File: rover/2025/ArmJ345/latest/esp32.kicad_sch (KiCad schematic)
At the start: 15 parts, among them SW1 SW-PTS815SJM250SMTRLFS, SW2 SW-PTS815SJM250SMTRLFS, U7 ESP32-S3-WROVER

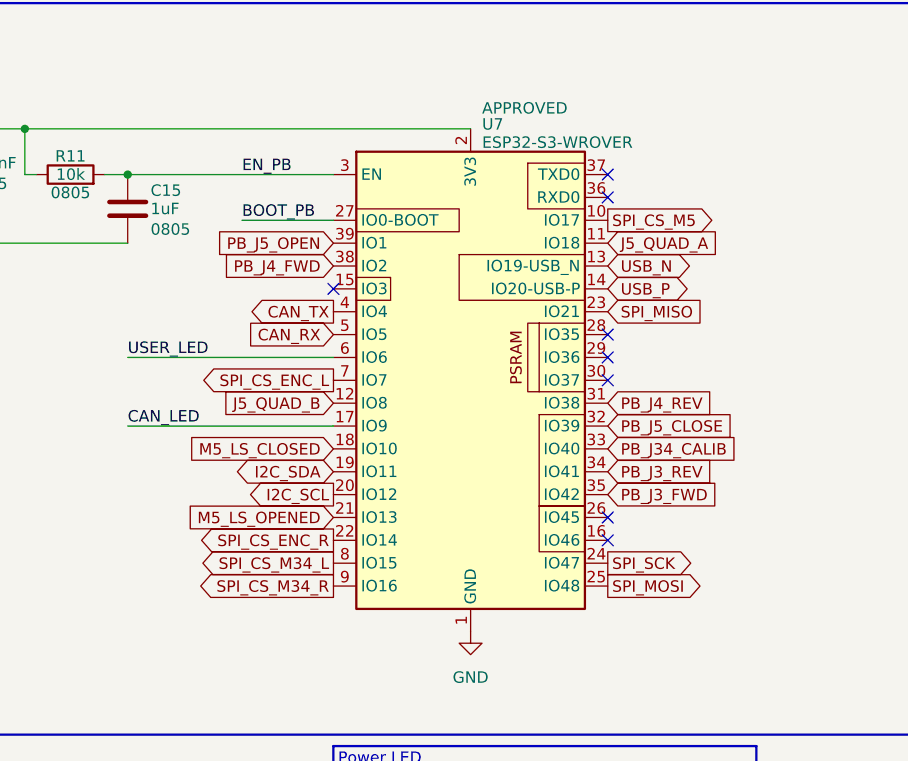
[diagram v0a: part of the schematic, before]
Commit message: armj345 fixes
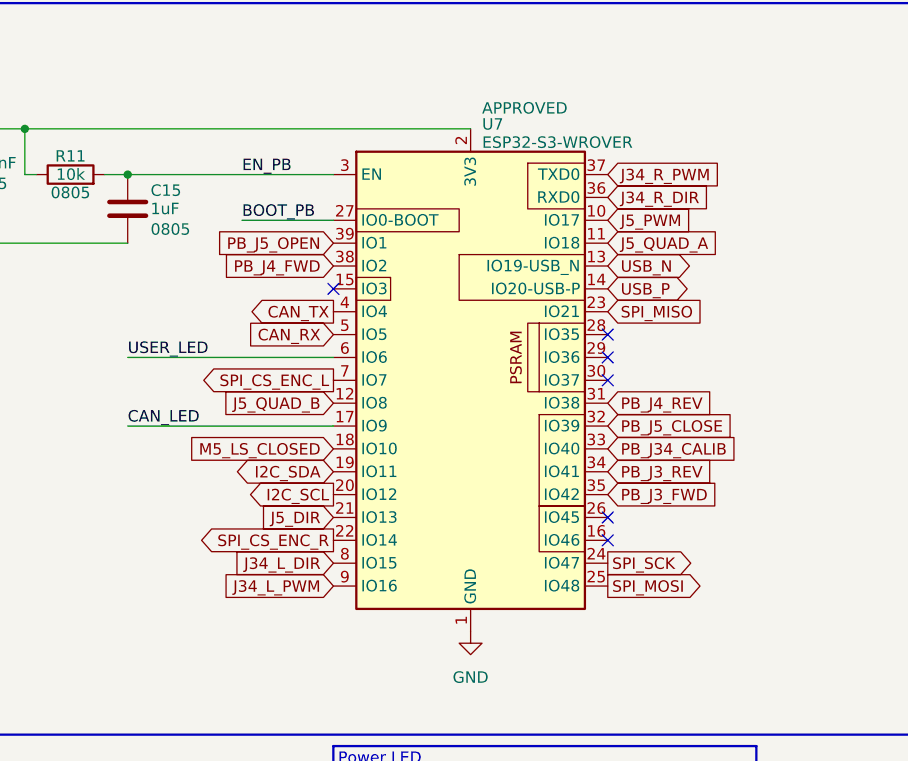
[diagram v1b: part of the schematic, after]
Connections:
- net J34_R_DIR: now reaches U7.36 (RXD0)
- net J34_R_PWM: now reaches U7.37 (TXD0)
- net M5_LS_OPENED renamed J5_DIR
- net SPI_CS_M34_L renamed J34_L_DIR
- net SPI_CS_M34_R renamed J34_L_PWM
- net SPI_CS_M5 renamed J5_PWM
- no-connect marks 8 -> 6
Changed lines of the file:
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@@
-	)
-	(no_connect
-		(at 116.84 31.75)
-	)
-	(no_connect
-		(at 116.84 34.29)
 	)
 	(no_connect
@@
 		)
 	)
-	(global_label "SPI_CS_M5"
-		(shape output)
+	(global_label "J5_PWM"
+		(shape input)
 		(at 116.84 36.83 0)
 		(fields_autoplaced yes)
@@
 		)
 		(property "Intersheetrefs" "${INTERSHEET_REFS}"
-			(at 129.9851 36.83 0)
+			(at 127.1427 36.83 0)
 			(effects
 				(font
@@
 		)
 	)
+	(global_label "J34_L_PWM"
+		(shape input)
+		(at 86.36 77.47 180)
+		(fields_autoplaced yes)
+		(effects
+			(font
+				(size 1.27 1.27)
+			)
+			(justify right)
+		)
+		(property "Intersheetrefs" "${INTERSHEET_REFS}"
+			(at 72.8521 77.47 0)
+			(effects
+				(font
+					(size 1.27 1.27)
+				)
+				(justify right)
+				(hide yes)
+			)
+		)
+	)
 	(global_label "SPI_CS_ENC_L"
 		(shape output)
@@
 		)
 	)
+	(global_label "J5_DIR"
+		(shape input)
+		(at 86.36 69.85 180)
+		(fields_autoplaced yes)
+		(effects
+			(font
+				(size 1.27 1.27)
+			)
+			(justify right)
+		)
+		(property "Intersheetrefs" "${INTERSHEET_REFS}"
+			(at 77.0853 69.85 0)
+			(effects
+				(font
+					(size 1.27 1.27)
+				)
+				(justify right)
+				(hide yes)
+			)
+		)
+	)
 	(global_label "PB_J5_OPEN"
 		(shape input)
@@
 		)
 	)
+	(global_label "J34_R_PWM"
+		(shape input)
+		(at 116.84 31.75 0)
+		(fields_autoplaced yes)
+		(effects
+			(font
+				(size 1.27 1.27)
+			)
+			(justify left)
+		)
+		(property "Intersheetrefs" "${INTERSHEET_REFS}"
+			(at 130.5898 31.75 0)
+			(effects
+				(font
+					(size 1.27 1.27)
+				)
+				(justify left)
+				(hide yes)
+			)
+		)
+	)
 	(global_label "USB_P"
 		(shape bidirectional)
@@
 		)
 	)
+	(global_label "J34_L_DIR"
+		(shape input)
+		(at 86.36 74.93 180)
+		(fields_autoplaced yes)
+		(effects
+			(font
+				(size 1.27 1.27)
+			)
+			(justify right)
+		)
+		(property "Intersheetrefs" "${INTERSHEET_REFS}"
+			(at 73.8801 74.93 0)
+			(effects
+				(font
+					(size 1.27 1.27)
+				)
+				(justify right)
+				(hide yes)
+			)
+		)
+	)
 	(global_label "SPI_MISO"
 		(shape input)
@@
 		(property "Intersheetrefs" "${INTERSHEET_REFS}"
 			(at 128.4733 46.99 0)
+			(effects
+				(font
+					(size 1.27 1.27)
+				)
+				(justify left)
+				(hide yes)
+			)
+		)
+	)
+	(global_label "J34_R_DIR"
+		(shape input)
+		(at 116.84 34.29 0)
+		(fields_autoplaced yes)
+		(effects
+			(font
+				(size 1.27 1.27)
+			)
+			(justify left)
+		)
+		(property "Intersheetrefs" "${INTERSHEET_REFS}"
+			(at 129.5618 34.29 0)
 			(effects
 				(font
@@
 		)
 	)
-	(global_label "SPI_CS_M34_R"
-		(shape output)
-		(at 86.36 77.47 180)
-		(fields_autoplaced yes)
-		(effects
-			(font
-				(size 1.27 1.27)
-			)
-			(justify right)
-		)
-		(property "Intersheetrefs" "${INTERSHEET_REFS}"
-			(at 69.7678 77.47 0)
-			(effects
-				(font
-					(size 1.27 1.27)
-				)
-				(justify right)
-				(hide yes)
-			)
-		)
-	)
 	(global_label "I2C_SDA"
 		(shape bidirectional)
@@
 		)
 	)
-	(global_label "M5_LS_OPENED"
-		(shape input)
-		(at 86.36 69.85 180)
-		(fields_autoplaced yes)
-		(effects
-			(font
-				(size 1.27 1.27)
-				(thickness 0.1588)
-			)
-			(justify right)
-		)
-		(property "Intersheetrefs" "${INTERSHEET_REFS}"
-			(at 68.5661 69.85 0)
-			(effects
-				(font
-					(size 1.27 1.27)
-				)
-				(justify right)
-				(hide yes)
-			)
-		)
-	)
 	(global_label "CAN_RX"
 		(shape input)
@@
 			(effects
 				(font
-					(size 1.27 1.27)
-				)
-				(justify right)
-				(hide yes)
-			)
-		)
-	)
-	(global_label "SPI_CS_M34_L"
-		(shape output)
-		(at 86.36 74.93 180)
-		(fields_autoplaced yes)
-		(effects
-			(font
-				(size 1.27 1.27)
-			)
-			(justify right)
-		)
-		(property "Intersheetrefs" "${INTERSHEET_REFS}"
-			(at 70.0097 74.93 0)
-			(effects
-				(font
